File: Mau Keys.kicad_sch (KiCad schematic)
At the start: 2 parts

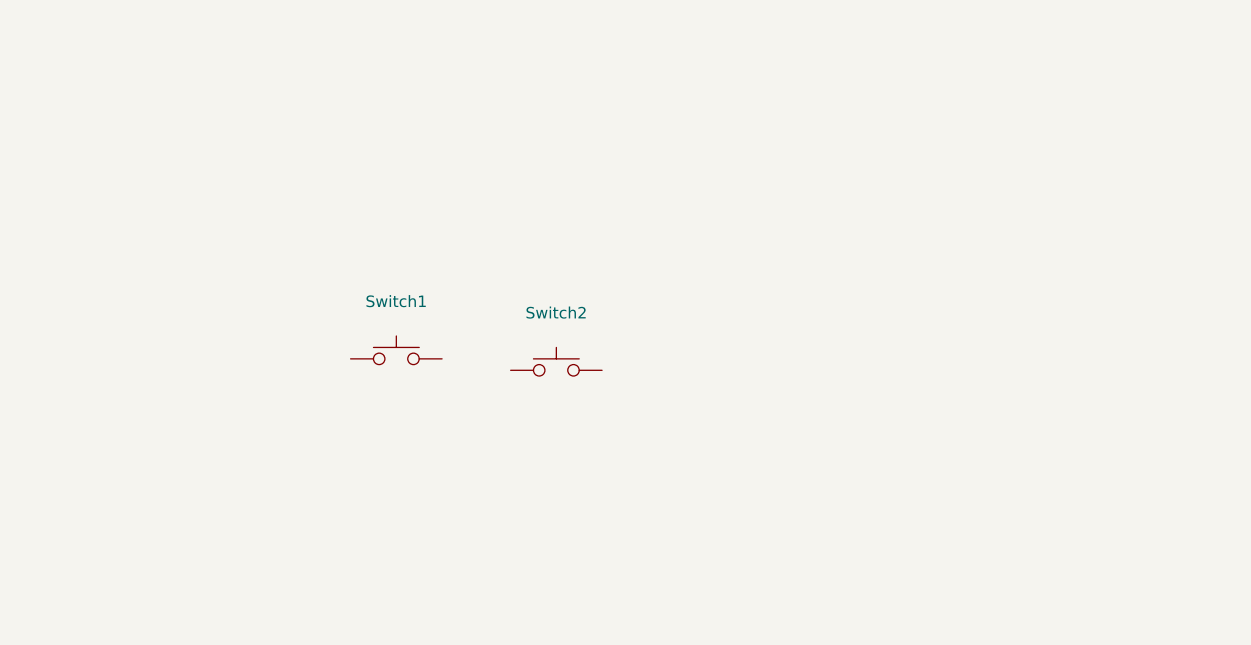
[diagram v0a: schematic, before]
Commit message: holaaa
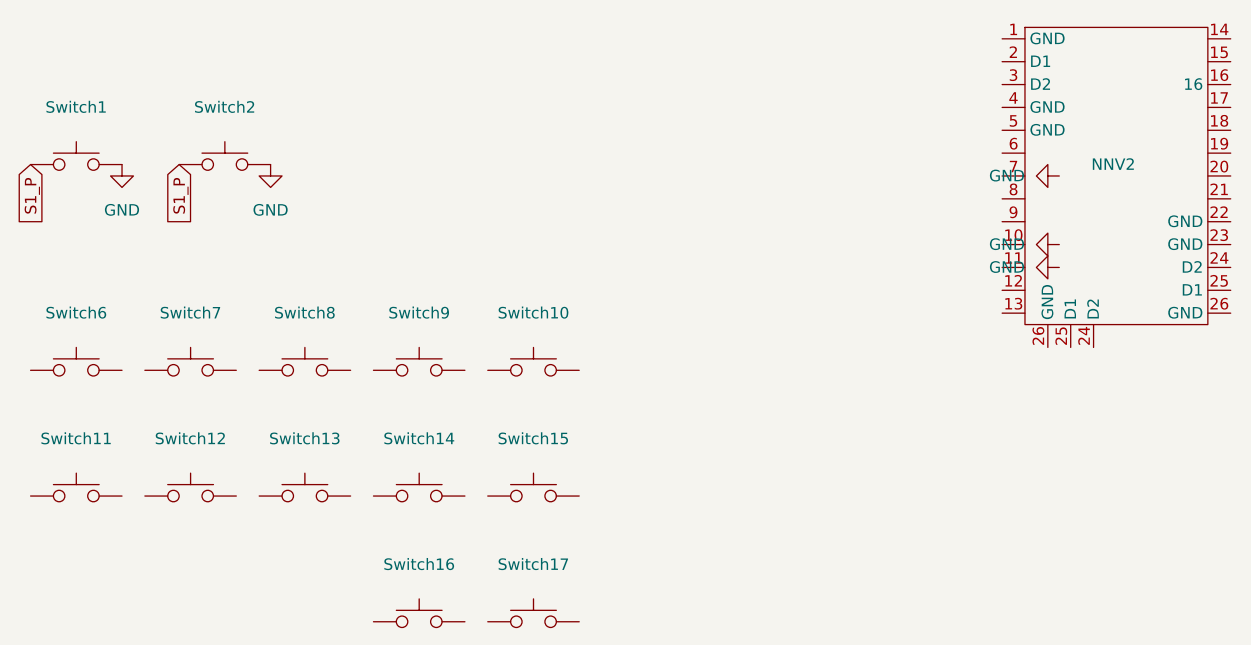
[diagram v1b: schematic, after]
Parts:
- added NNV2: ~, symbol MCC NNV2:NNano_v2
- added Switch10, Switch11, Switch12, Switch13, Switch14, Switch15, Switch16, Switch17, Switch6, Switch7, Switch8, Switch9: ~, Switches:keyswitch_cherrymx_alps_choc12_slots_1u, symbol Switches:Kailh_ChocV2_Switch
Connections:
- net S1_P: now reaches Switch1.1
- net S1_P: now also Switch2.1
- net GND: now reaches Switch1.2
- net GND: now also Switch2.2
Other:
- moved on the sheet: Switch1

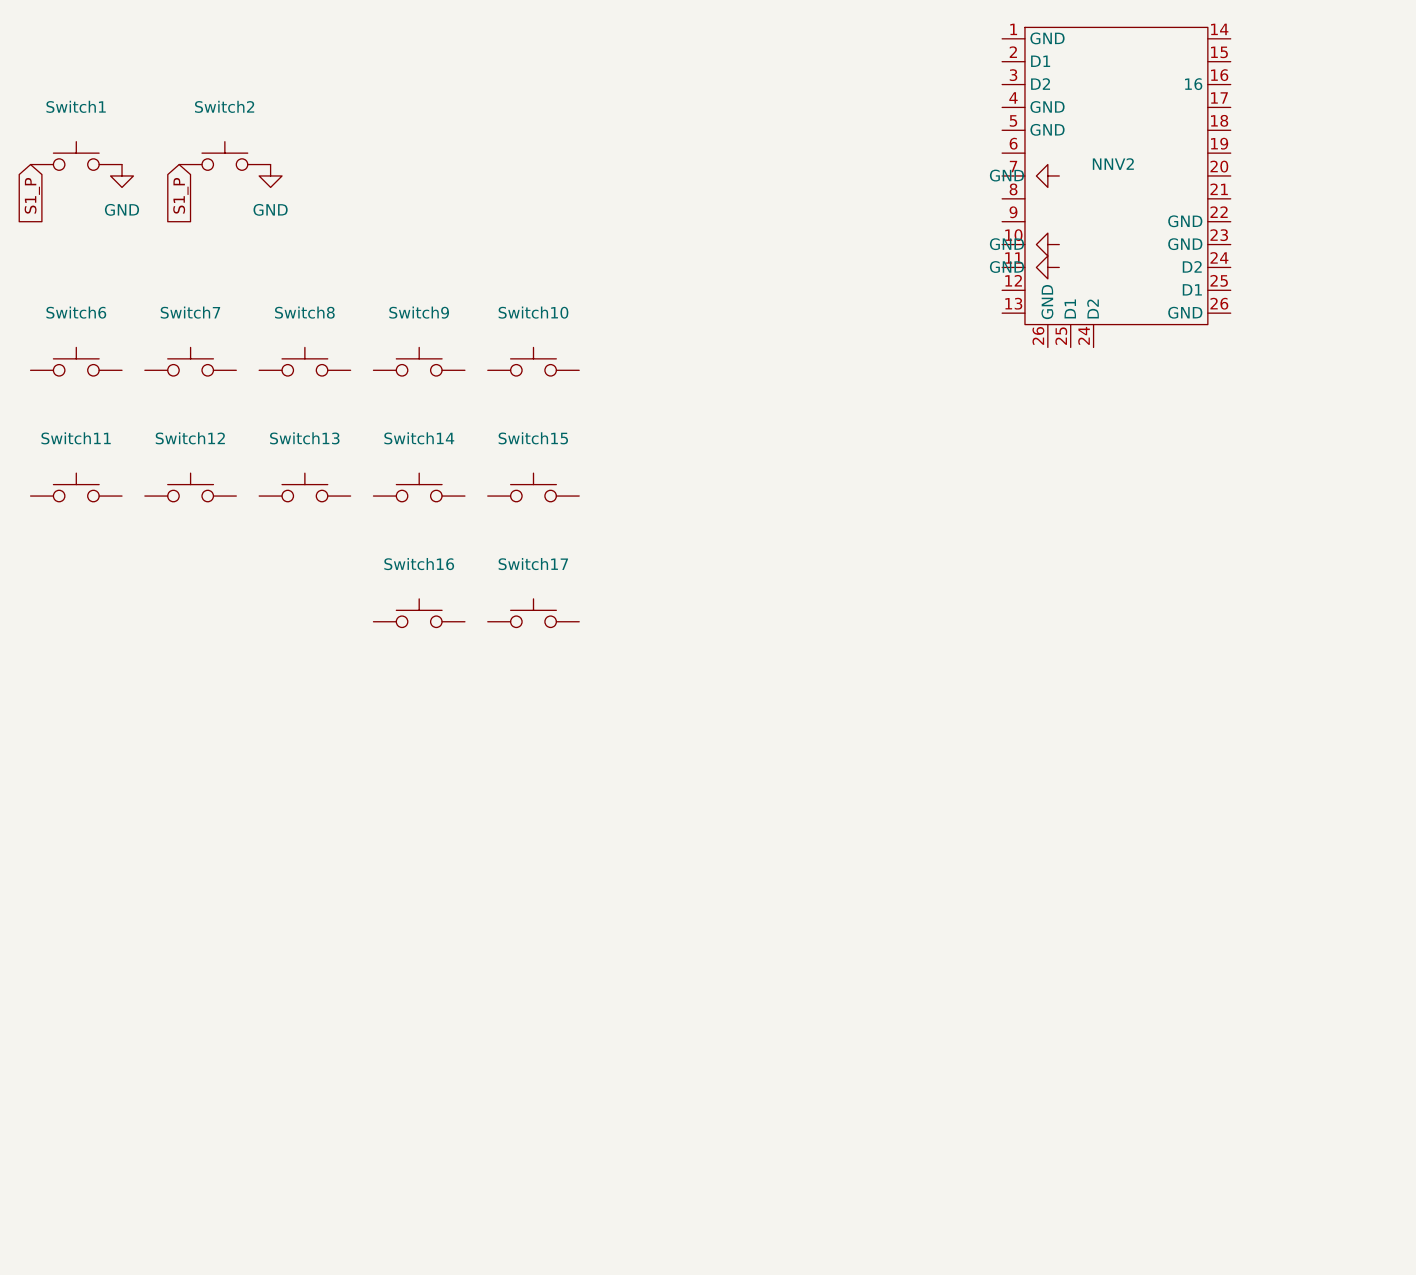
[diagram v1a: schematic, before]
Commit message: Initial traces
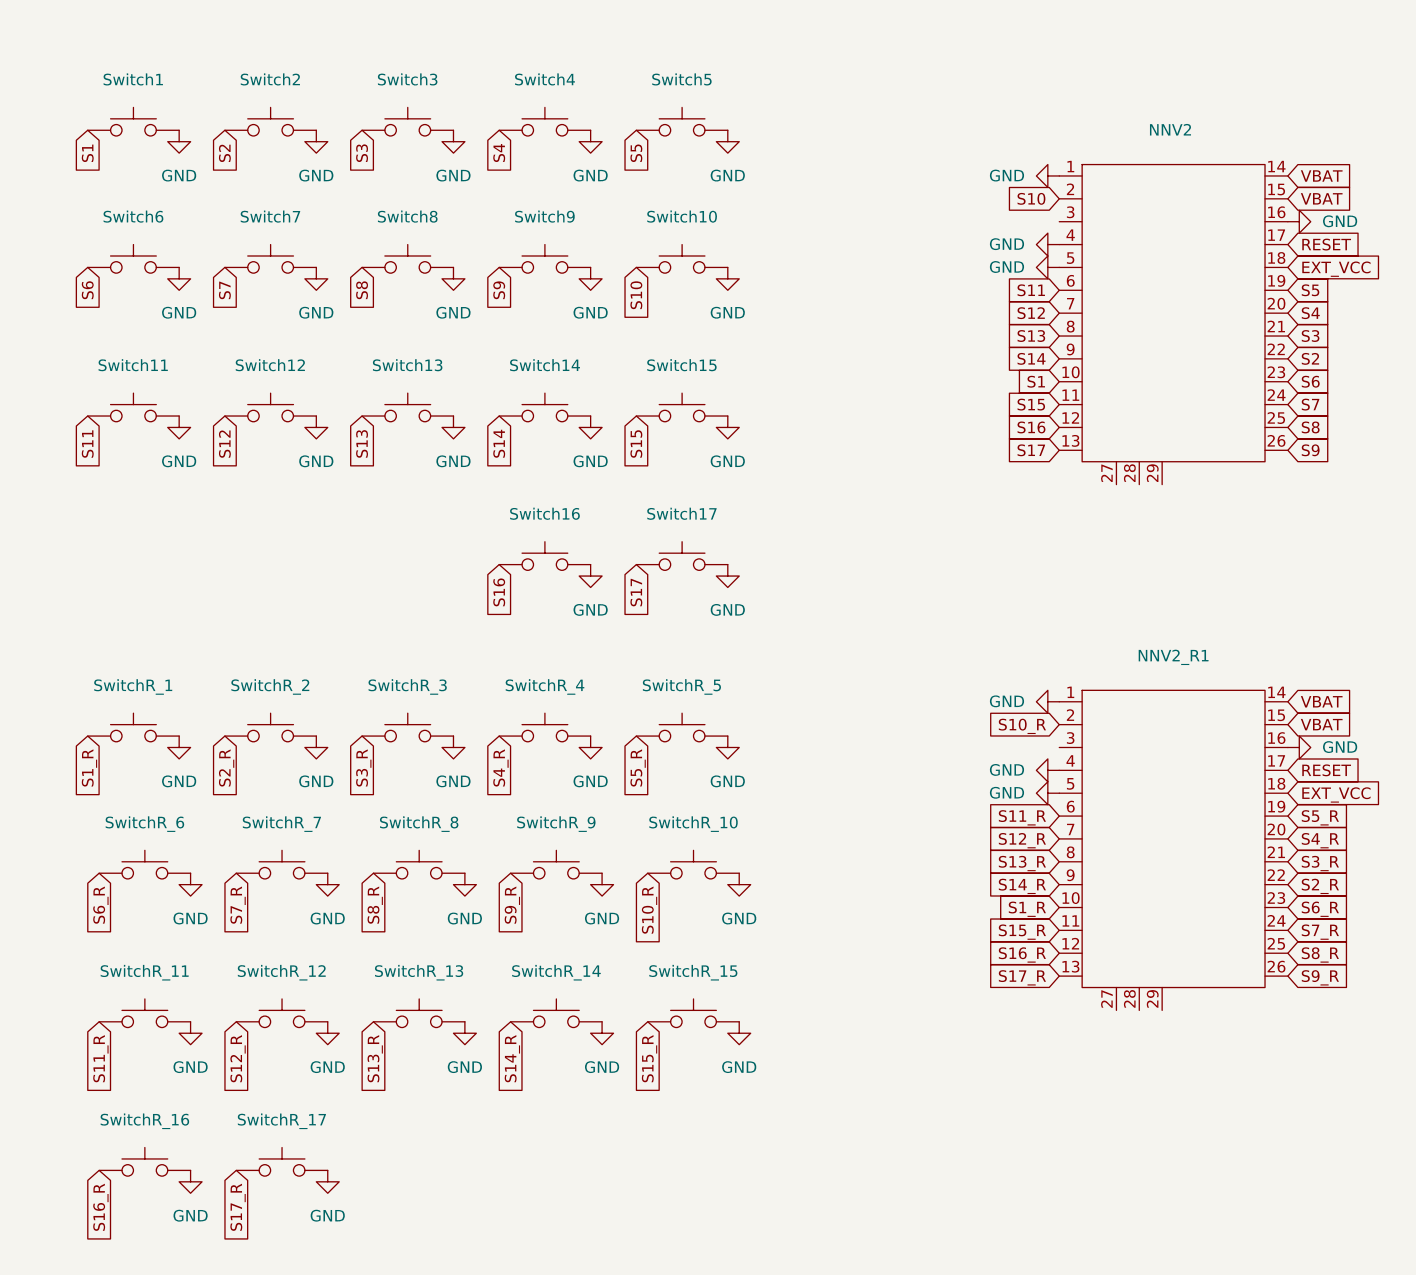
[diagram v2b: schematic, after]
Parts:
- added NNV2_R1: ~, Microcontroller:nice_nano, symbol MCC NNV2:NNano_v2
- added Switch3, Switch4, Switch5, SwitchR_1, SwitchR_10, SwitchR_11, SwitchR_12, SwitchR_13, SwitchR_14, SwitchR_15, SwitchR_16, SwitchR_17, SwitchR_2, SwitchR_3, SwitchR_4, SwitchR_5, SwitchR_6, SwitchR_7, SwitchR_8, SwitchR_9: ~, Switches:keyswitch_cherrymx_alps_choc12_slots_1u, symbol Switches:Kailh_ChocV2_Switch
- NNV2: footprint (none) -> Microcontroller:nice_nano
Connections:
- net GND: now also NNV2.1, NNV2.16, NNV2.4, NNV2.5, Switch10.2, Switch11.2, Switch12.2, Switch13.2, Switch14.2, Switch15.2, Switch16.2, Switch17.2, Switch6.2, Switch7.2, Switch8.2, Switch9.2, NNV2_R1.1, NNV2_R1.16, NNV2_R1.4, NNV2_R1.5, Switch3.2, Switch4.2, Switch5.2, SwitchR_1.2, SwitchR_10.2, SwitchR_11.2, SwitchR_12.2, SwitchR_13.2, SwitchR_14.2, SwitchR_15.2, SwitchR_16.2, SwitchR_17.2, SwitchR_2.2, SwitchR_3.2, SwitchR_4.2, SwitchR_5.2, SwitchR_6.2, SwitchR_7.2, SwitchR_8.2, SwitchR_9.2
- net S9: now reaches Switch9.1
- net S9: now also NNV2.26
- net S12: now reaches Switch12.1
- net S12: now also NNV2.7
- net S15: now reaches Switch15.1
- net S15: now also NNV2.11
- net S11: now reaches Switch11.1
- net S11: now also NNV2.6
- net S13: now reaches Switch13.1
- net S13: now also NNV2.8
- net S17: now reaches Switch17.1
- net S17: now also NNV2.13
- net S10: now reaches Switch10.1
- net S10: now also NNV2.2
- net S16: now reaches Switch16.1
- net S16: now also NNV2.12
- net S1: now reaches NNV2.10
- net S1: now also Switch1.1
- net VBAT: now reaches NNV2.14
- net VBAT: now also NNV2.15, NNV2_R1.14, NNV2_R1.15
- net RESET: now reaches NNV2.17
- net RESET: now also NNV2_R1.17
- net EXT_VCC: now reaches NNV2.18
- net EXT_VCC: now also NNV2_R1.18
- net S5: now reaches NNV2.19
- net S5: now also Switch5.1
- net S4: now reaches NNV2.20
- net S4: now also Switch4.1
- net S3: now reaches NNV2.21
- net S3: now also Switch3.1
- net S2: now reaches NNV2.22
- net S2: now also Switch2.1
- net S6: now reaches NNV2.23
- net S6: now also Switch6.1
- net S7: now reaches NNV2.24
- net S7: now also Switch7.1
- net S8: now reaches NNV2.25
- net S8: now also Switch8.1
- net S14: now reaches NNV2.9
- net S14: now also Switch14.1
- removed net S1_P: Switch1.1, Switch2.1
- new net S10_R: NNV2_R1.2, SwitchR_10.1
- new net S11_R: NNV2_R1.6, SwitchR_11.1
- new net S12_R: NNV2_R1.7, SwitchR_12.1
- new net S13_R: NNV2_R1.8, SwitchR_13.1
- new net S14_R: NNV2_R1.9, SwitchR_14.1
- new net S15_R: NNV2_R1.11, SwitchR_15.1
- new net S16_R: NNV2_R1.12, SwitchR_16.1
- new net S17_R: NNV2_R1.13, SwitchR_17.1
- new net S1_R: NNV2_R1.10, SwitchR_1.1
- new net S2_R: NNV2_R1.22, SwitchR_2.1
- new net S3_R: NNV2_R1.21, SwitchR_3.1
- new net S4_R: NNV2_R1.20, SwitchR_4.1
- new net S5_R: NNV2_R1.19, SwitchR_5.1
- new net S6_R: NNV2_R1.23, SwitchR_6.1
- new net S7_R: NNV2_R1.24, SwitchR_7.1
- new net S8_R: NNV2_R1.25, SwitchR_8.1
- new net S9_R: NNV2_R1.26, SwitchR_9.1
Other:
- moved on the sheet: Switch1
